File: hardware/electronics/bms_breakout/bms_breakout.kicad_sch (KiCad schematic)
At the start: 66 parts, among them J1 Conn_01x03_Socket, Q1 BUK961R6-40E, Q2 VAL, Q3 VAL, U1 BQ76905, U2 BQ25798RQMR

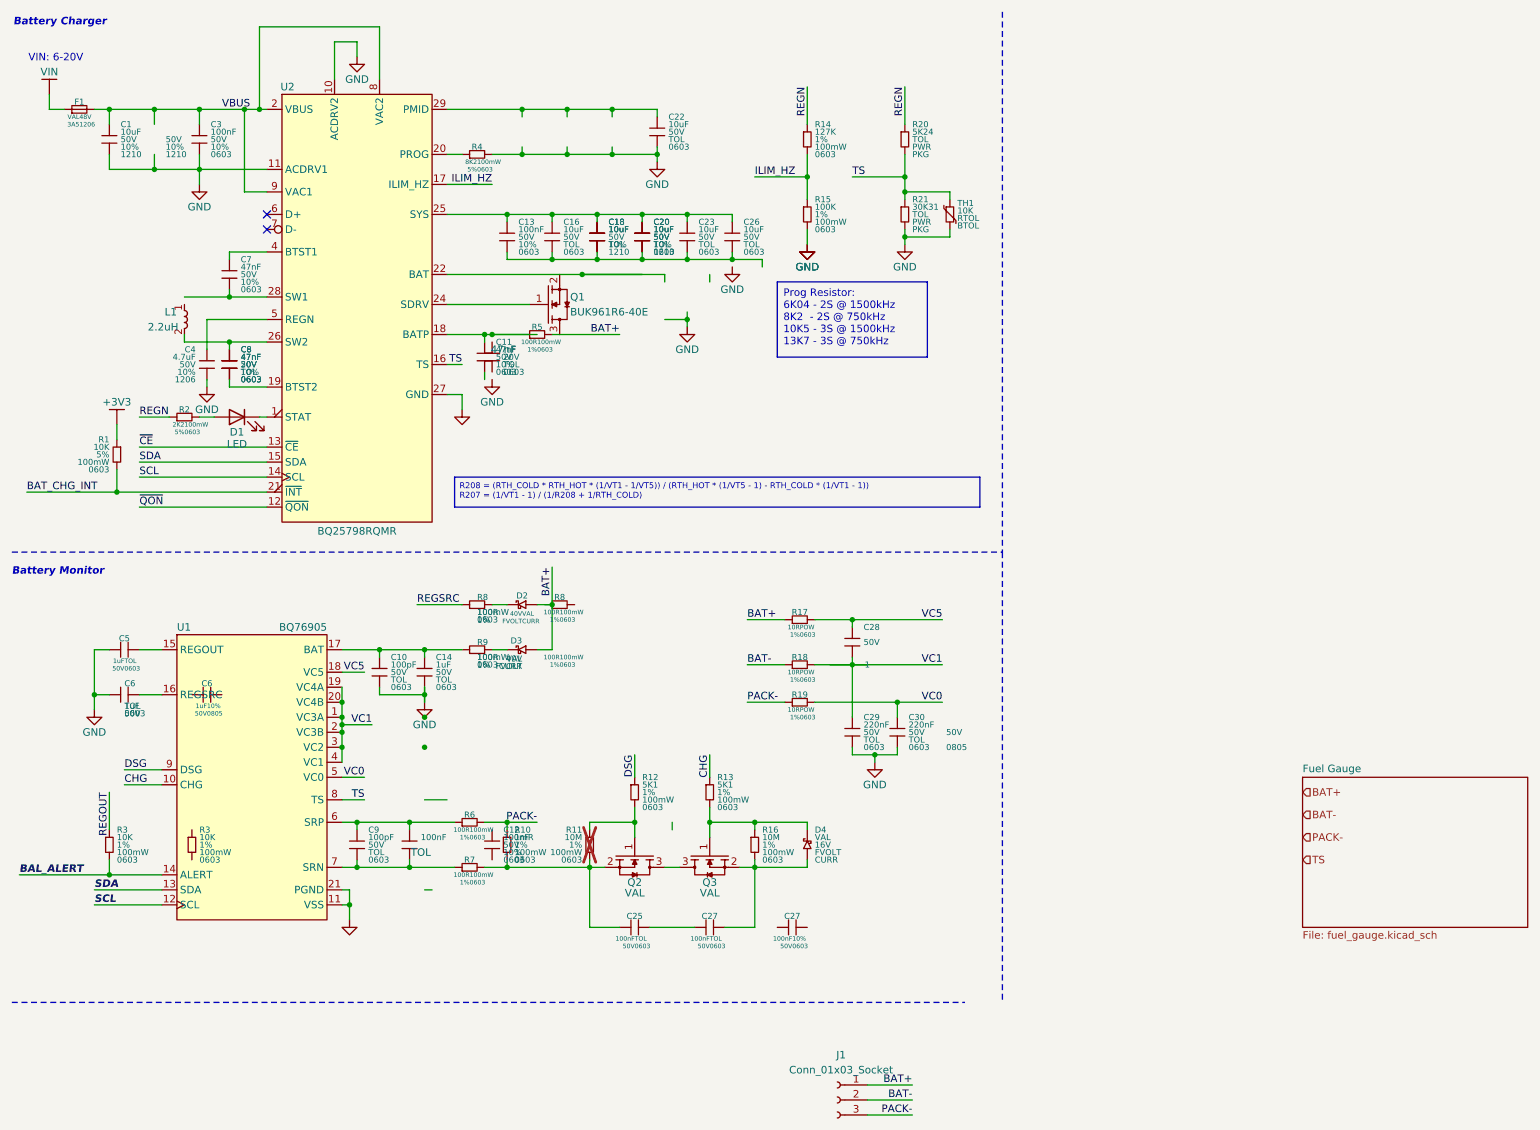
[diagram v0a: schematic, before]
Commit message: fixed drawing sheet ref
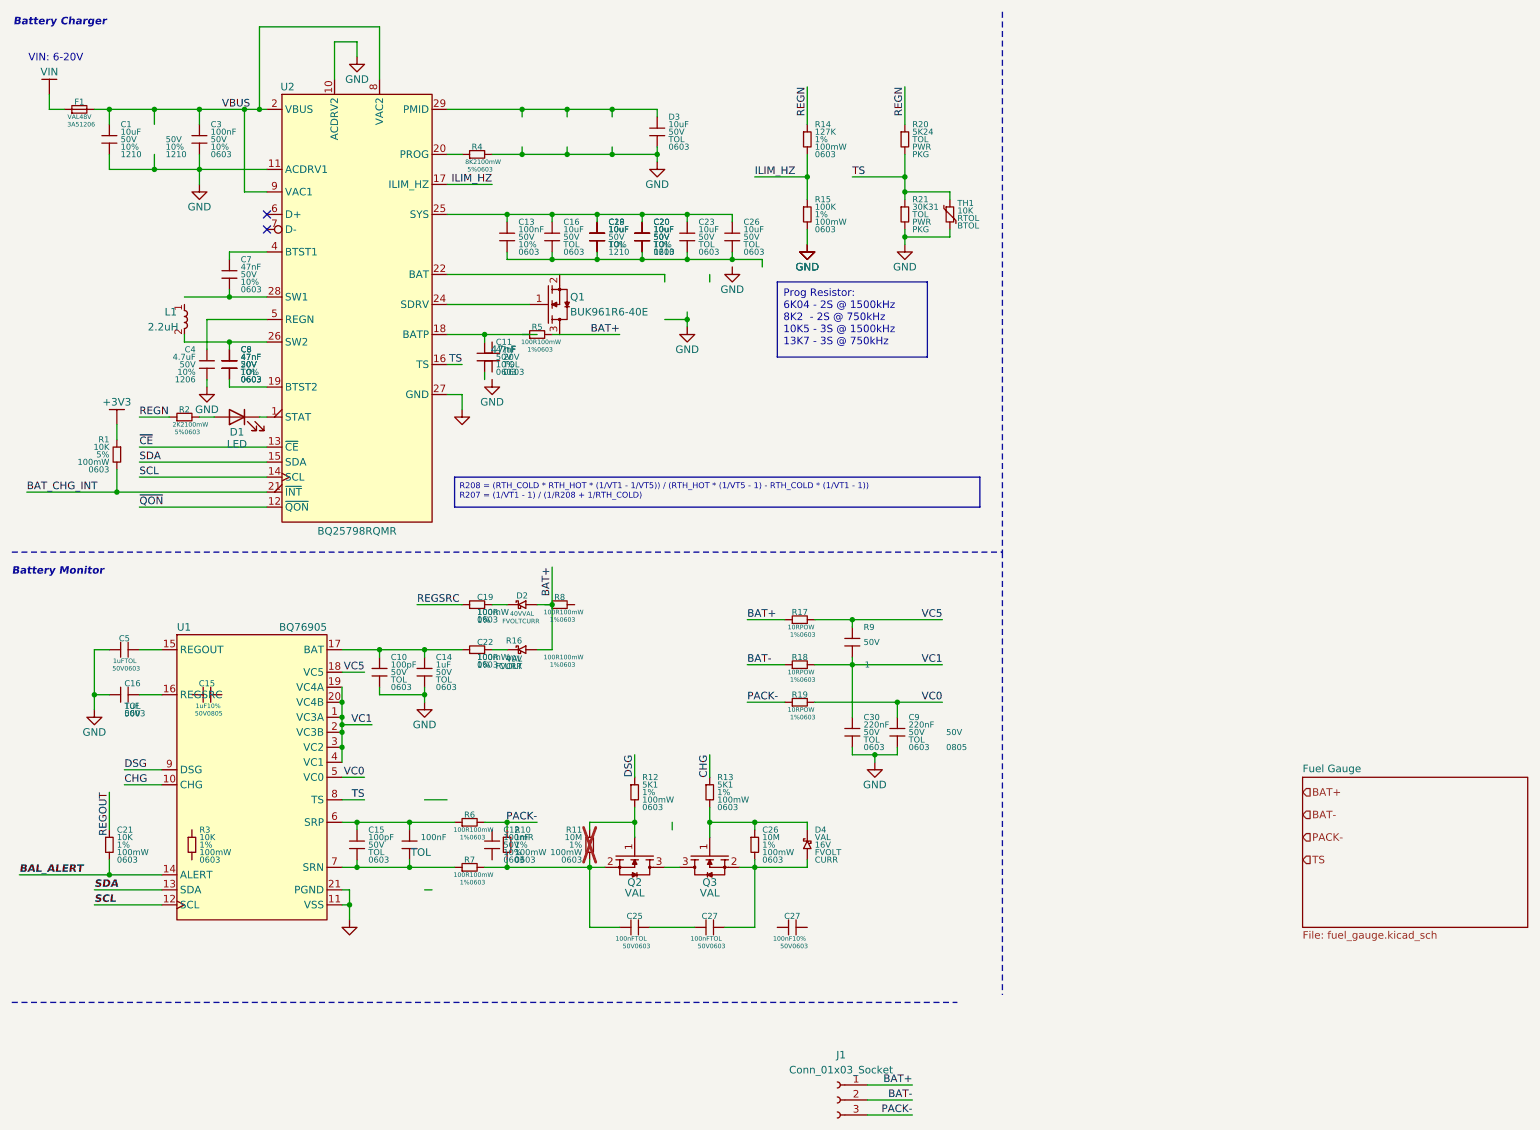
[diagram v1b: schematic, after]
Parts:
- added R3: 10K, DSE-Resistors-SMD:RESC160X80X55L30N, symbol DSE-Passives:R
- C21: renamed from R3; footprint DSE-Resistors-SMD:RESC160X80X55L30N -> (none); populate (none) -> 1
- renumbered C12 to #PWR02, C9 to C15, C6 to C15, C6 to C16, R8 to C19, R9 to C22, R16 to C26, C18 to C29, C29 to C30, C30 to C9, C22 to D3, D3 to R16, C28 to R9
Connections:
- net at C11.1, U2.18 (BATP): no longer R5.1
